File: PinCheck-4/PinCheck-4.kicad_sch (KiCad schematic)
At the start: 18 parts

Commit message: Daily sync 2025-08-30 21:30
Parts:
- D1, D3, D4, D5, D6: footprint LED_THT:LED_D3.0mm_Clear -> LED_SMD:LED_0805_2012Metric; Manufacturer Part No L-934GD -> KP-2012MGC
- D2: footprint LED_THT:LED_D3.0mm_Clear -> LED_SMD:LED_0805_2012Metric; Manufacturer Part No L-934ND -> KP-2012SECK
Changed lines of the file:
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@@
 			)
 		)
-		(property "Footprint" "LED_THT:LED_D3.0mm_Clear"
+		(property "Footprint" "LED_SMD:LED_0805_2012Metric"
 			(at 21.59 168.91 0)
 			(effects
@@
 			)
 		)
-		(property "Description" "LED, Low Power, Green, Through Hole, T-1 (3mm), 20 mA, 2.2 V, 568 nm"
+		(property "Description" "LED, Low Power, Green, SMD, 0805 [2012 Metric], 20 mA, 2.1 V, 570 nm"
 			(at 21.59 168.91 0)
 			(effects
@@
 			)
 		)
-		(property "Manufacturer Part No" "L-934GD"
+		(property "Manufacturer Part No" "KP-2012MGC"
 			(at 21.59 168.91 90)
 			(effects
@@
 			)
 		)
-		(property "Footprint" "LED_THT:LED_D3.0mm_Clear"
+		(property "Footprint" "LED_SMD:LED_0805_2012Metric"
 			(at 72.39 168.91 0)
 			(effects
@@
 			)
 		)
-		(property "Description" "LED, Low Power, Green, Through Hole, T-1 (3mm), 20 mA, 2.2 V, 568 nm"
+		(property "Description" "LED, Low Power, Green, SMD, 0805 [2012 Metric], 20 mA, 2.1 V, 570 nm"
 			(at 72.39 168.91 0)
 			(effects
@@
 			)
 		)
-		(property "Manufacturer Part No" "L-934GD"
+		(property "Manufacturer Part No" "KP-2012MGC"
 			(at 72.39 168.91 90)
 			(effects
@@
 			)
 		)
-		(property "Footprint" "LED_THT:LED_D3.0mm_Clear"
+		(property "Footprint" "LED_SMD:LED_0805_2012Metric"
 			(at 62.23 168.91 0)
 			(effects
@@
 			)
 		)
-		(property "Description" "LED, Low Power, Green, Through Hole, T-1 (3mm), 20 mA, 2.2 V, 568 nm"
+		(property "Description" "LED, Low Power, Green, SMD, 0805 [2012 Metric], 20 mA, 2.1 V, 570 nm"
 			(at 62.23 168.91 0)
 			(effects
@@
 			)
 		)
-		(property "Manufacturer Part No" "L-934GD"
+		(property "Manufacturer Part No" "KP-2012MGC"
 			(at 62.23 168.91 90)
 			(effects
@@
 			)
 		)
-		(property "Footprint" "LED_THT:LED_D3.0mm_Clear"
+		(property "Footprint" "LED_SMD:LED_0805_2012Metric"
 			(at 41.91 168.91 0)
 			(effects
@@
 			)
 		)
-		(property "Description" "LED, Low Power, Green, Through Hole, T-1 (3mm), 20 mA, 2.2 V, 568 nm"
+		(property "Description" "LED, Low Power, Green, SMD, 0805 [2012 Metric], 20 mA, 2.1 V, 570 nm"
 			(at 41.91 168.91 0)
 			(effects
@@
 			)
 		)
-		(property "Manufacturer Part No" "L-934GD"
+		(property "Manufacturer Part No" "KP-2012MGC"
 			(at 41.91 168.91 90)
 			(effects
@@
 			)
 		)
-		(property "Footprint" "LED_THT:LED_D3.0mm_Clear"
+		(property "Footprint" "LED_SMD:LED_0805_2012Metric"
 			(at 31.75 168.91 0)
 			(effects
@@
 			)
 		)
-		(property "Description" "LED, Low Power, Orange, Through Hole, T-1 (3mm), 20 mA, 2.05 V, 610 nm"
+		(property "Description" "LED, Low Power, Orange, SMD, 0805 [2012 Metric], 20 mA, 2.1 V, 601 nm"
 			(at 31.75 168.91 0)
 			(effects
@@
 			)
 		)
-		(property "Manufacturer Part No" "L-934ND"
+		(property "Manufacturer Part No" "KP-2012SECK"
 			(at 31.75 168.91 90)
 			(effects
@@
 			)
 		)
-		(property "Footprint" "LED_THT:LED_D3.0mm_Clear"
+		(property "Footprint" "LED_SMD:LED_0805_2012Metric"
 			(at 52.07 168.91 0)
 			(effects
@@
 			)
 		)
-		(property "Description" "LED, Low Power, Green, Through Hole, T-1 (3mm), 20 mA, 2.2 V, 568 nm"
+		(property "Description" "LED, Low Power, Green, SMD, 0805 [2012 Metric], 20 mA, 2.1 V, 570 nm"
 			(at 52.07 168.91 0)
 			(effects
@@
 			)
 		)
-		(property "Manufacturer Part No" "L-934GD"
+		(property "Manufacturer Part No" "KP-2012MGC"
 			(at 52.07 168.91 90)
 			(effects

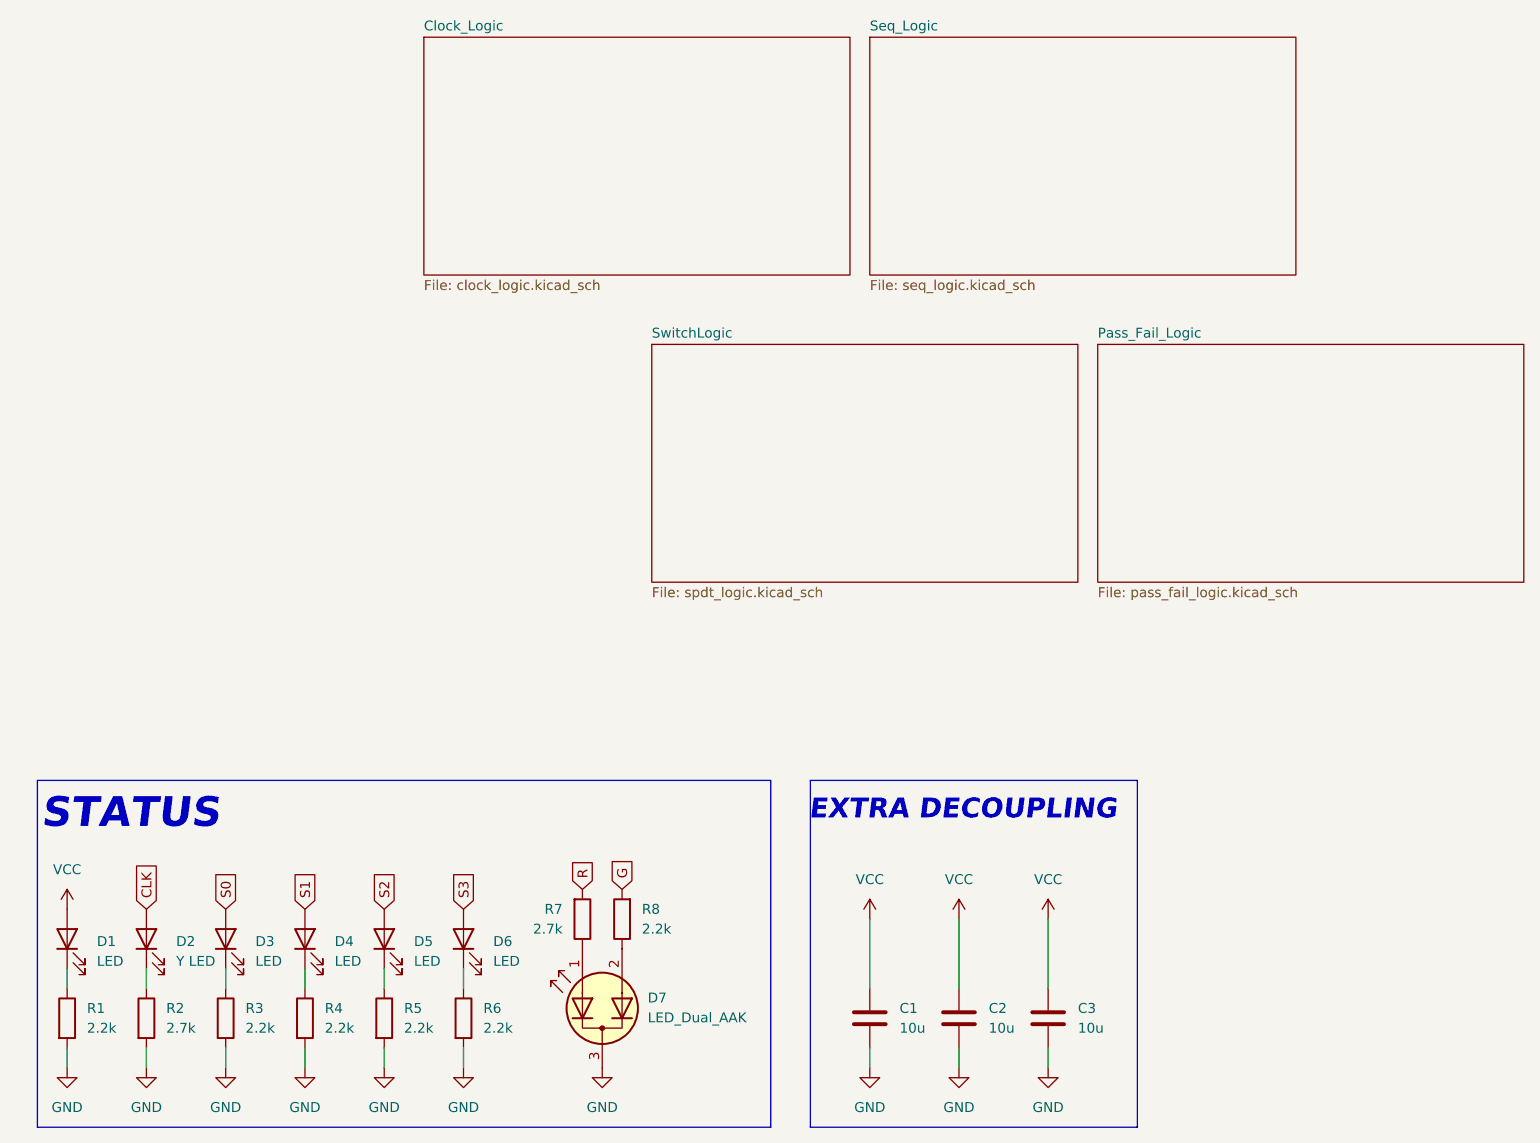
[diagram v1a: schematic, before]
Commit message: Daily sync 2025-08-31 12:14
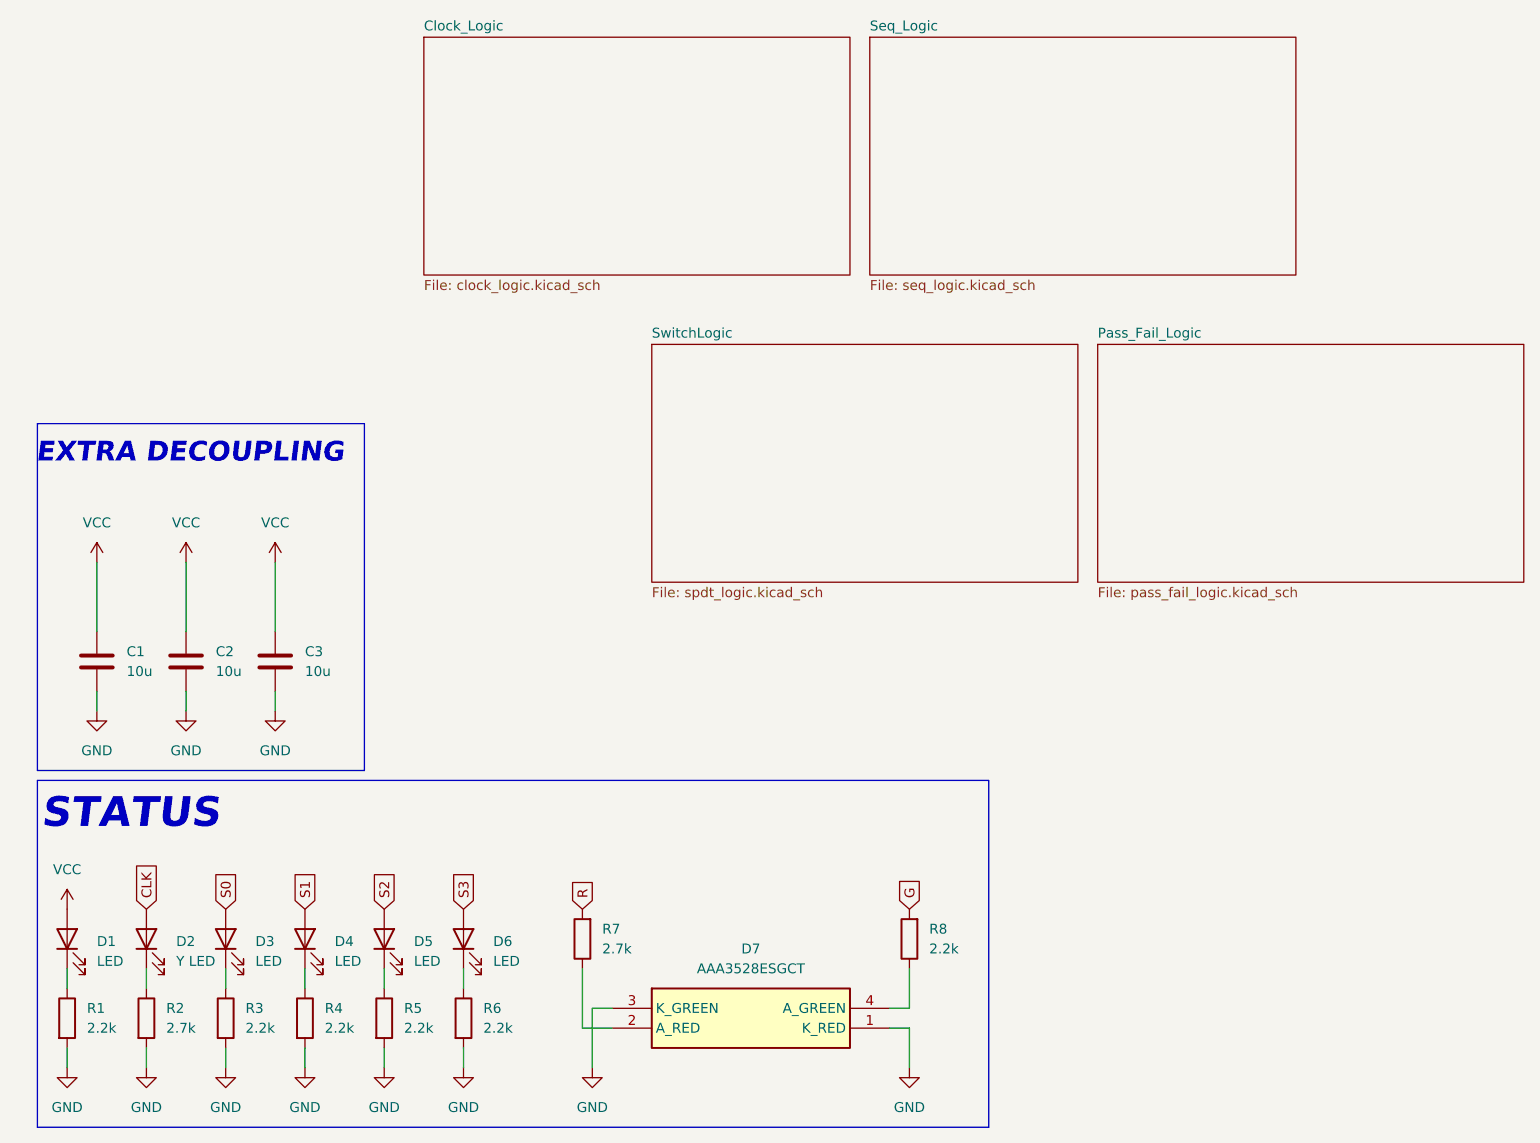
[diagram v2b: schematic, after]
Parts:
- removed D7: LED_Dual_AAK, LED_THT:LED_D3.0mm-3, symbol Device:LED_Dual_AAK
- added D7: AAA3528ESGCT, LED_SMD:AAA3528ESGCT, symbol Device:AAA3528ESGCT
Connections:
- net GND: now also D7.1 (K_RED), D7.3 (K_GREEN)
- net at R7.1: now also D7.2 (A_RED)
- net at R8.1: now also D7.4 (A_GREEN)
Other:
- moved on the sheet: C1, C2, C3, R7, R8
